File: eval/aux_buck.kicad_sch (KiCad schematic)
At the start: 14 parts, among them U1 AP63205WU-7, U10 TPS7A2033PDBVR, U12 TPS7A2033PDBVR

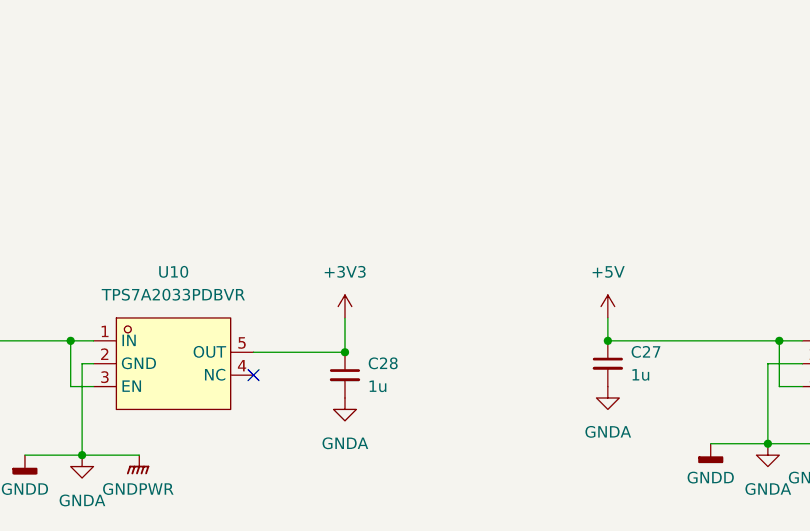
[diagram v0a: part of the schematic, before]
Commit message: [layout] 50*100mm, without trace
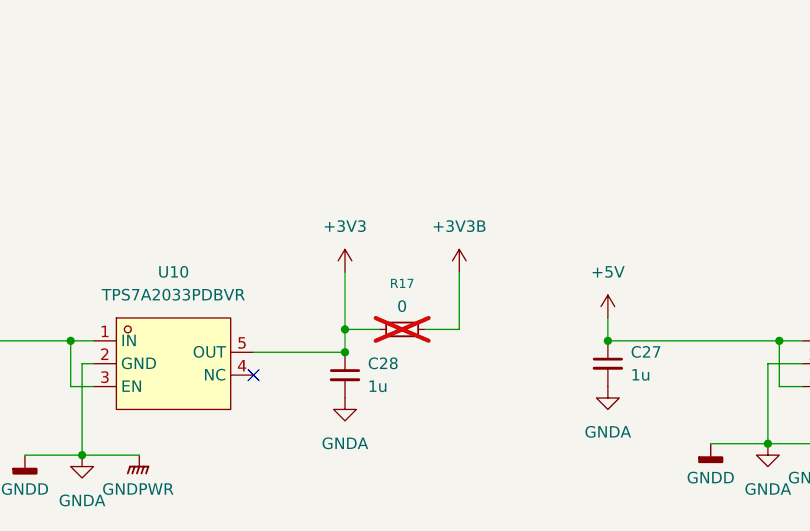
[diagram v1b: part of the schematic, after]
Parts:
- added R17: 0, symbol Device:R_Small
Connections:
- net +3V3: now also R17.1
- net +3V3B: now also R17.2
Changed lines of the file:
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@@
 	)
 	(junction
+		(at 91.44 118.11)
+		(diameter 0)
+		(color 0 0 0 0)
+	)
+	(junction
 		(at 139.7 119.38)
 		(diameter 0)
@@
 	(wire
 		(pts
-			(xy 91.44 116.84) (xy 91.44 120.65)
+			(xy 91.44 111.76) (xy 91.44 118.11)
 		)
 		(stroke
@@
 	(wire
 		(pts
+			(xy 104.14 118.11) (xy 100.33 118.11)
+		)
+		(stroke
+			(width 0)
+			(type default)
+		)
+	)
+	(wire
+		(pts
 			(xy 97.79 60.96) (xy 102.87 60.96)
 		)
@@
 	(wire
 		(pts
+			(xy 104.14 111.76) (xy 104.14 118.11)
+		)
+		(stroke
+			(width 0)
+			(type default)
+		)
+	)
+	(wire
+		(pts
 			(xy 132.08 67.31) (xy 132.08 66.04)
 		)
@@
 	(wire
 		(pts
+			(xy 91.44 118.11) (xy 91.44 120.65)
+		)
+		(stroke
+			(width 0)
+			(type default)
+		)
+	)
+	(wire
+		(pts
 			(xy 102.87 60.96) (xy 105.41 60.96)
 		)
@@
 	(wire
 		(pts
+			(xy 95.25 118.11) (xy 91.44 118.11)
+		)
+		(stroke
+			(width 0)
+			(type default)
+		)
+	)
+	(wire
+		(pts
 			(xy 171.45 120.65) (xy 160.02 120.65)
 		)
@@
 	)
 	(symbol
+		(lib_id "Device:R_Small")
+		(at 97.79 118.11 90)
+		(unit 1)
+		(body_style 1)
+		(exclude_from_sim no)
+		(in_bom yes)
+		(on_board yes)
+		(in_pos_files yes)
+		(dnp yes)
+		(fields_autoplaced yes)
+		(property "Reference" "R17"
+			(at 97.79 113.03 90)
+			(show_name no)
+			(do_not_autoplace no)
+			(effects
+				(font
+					(size 1.016 1.016)
+				)
+			)
+		)
+		(property "Value" "0"
+			(at 97.79 115.57 90)
+			(show_name no)
+			(do_not_autoplace no)
+			(effects
+				(font
+					(size 1.27 1.27)
+				)
+			)
+		)
+		(property "Footprint" ""
+			(at 97.79 118.11 0)
+			(hide yes)
+			(show_name no)
+			(do_not_autoplace no)
+			(effects
+				(font
+					(size 1.27 1.27)
+				)
+			)
+		)
+		(property "Datasheet" ""
+			(at 97.79 118.11 0)
+			(hide yes)
+			(show_name no)
+			(do_not_autoplace no)
+			(effects
+				(font
+					(size 1.27 1.27)
+				)
+			)
+		)
+		(property "Description" "Resistor, small symbol"
+			(at 97.79 118.11 0)
+			(hide yes)
+			(show_name no)
+			(do_not_autoplace no)
+			(effects
+				(font
+					(size 1.27 1.27)
+				)
+			)
+		)
+		(pin "1"
+		)
+		(pin "2"
+		)
+		(instances
+			(project "eval"
+				(path "/8b023652-20db-48ce-ad53-bc2d9a4e5dd4/e5450d34-e34e-454c-8387-40410830d96b"
+					(reference "R17")
+					(unit 1)
+				)
+			)
+		)
+	)
+	(symbol
 		(lib_id "power:+5V")
 		(at 7.1264 11.1816 0)
@@
 	)
 	(symbol
+		(lib_id "power:+3V3")
+		(at 104.14 111.76 0)
+		(unit 1)
+		(body_style 1)
+		(exclude_from_sim no)
+		(in_bom yes)
+		(on_board yes)
+		(in_pos_files yes)
+		(dnp no)
+		(fields_autoplaced yes)
+		(property "Reference" "#PWR0135"
+			(at 104.14 115.57 0)
+			(hide yes)
+			(show_name no)
+			(do_not_autoplace no)
+			(effects
+				(font
+					(size 1.27 1.27)
+				)
+			)
+		)
+		(property "Value" "+3V3B"
+			(at 104.14 106.68 0)
+			(show_name no)
+			(do_not_autoplace no)
+			(effects
+				(font
+					(size 1.27 1.27)
+				)
+			)
+		)
+		(property "Footprint" ""
+			(at 104.14 111.76 0)
+			(hide yes)
+			(show_name no)
+			(do_not_autoplace no)
+			(effects
+				(font
+					(size 1.27 1.27)
+				)
+			)
+		)
+		(property "Datasheet" ""
+			(at 104.14 111.76 0)
+			(hide yes)
+			(show_name no)
+			(do_not_autoplace no)
+			(effects
+				(font
+					(size 1.27 1.27)
+				)
+			)
+		)
+		(property "Description" "Power symbol creates a global label with name \"+3V3\""
+			(at 104.14 111.76 0)
+			(hide yes)
+			(show_name no)
+			(do_not_autoplace no)
+			(effects
+				(font
+					(size 1.27 1.27)
+				)
+			)
+		)
+		(pin "1"
+		)
+		(instances
+			(project "eval"
+				(path "/8b023652-20db-48ce-ad53-bc2d9a4e5dd4/e5450d34-e34e-454c-8387-40410830d96b"
+					(reference "#PWR0135")
+					(unit 1)
+				)
+			)
+		)
+	)
+	(symbol
 		(lib_id "power:VBUS")
 		(at 52.07 53.34 0)
@@
 	(symbol
 		(lib_id "power:+3V3")
-		(at 91.44 116.84 0)
+		(at 91.44 111.76 0)
 		(unit 1)
 		(body_style 1)
@@
 		(fields_autoplaced yes)
 		(property "Reference" "#PWR038"
-			(at 91.44 120.65 0)
+			(at 91.44 115.57 0)
 			(hide yes)
 			(show_name no)
@@
 		)
 		(property "Value" "+3V3"
-			(at 91.44 111.76 0)
+			(at 91.44 106.68 0)
 			(show_name no)
 			(do_not_autoplace no)
@@
 		)
 		(property "Footprint" ""
-			(at 91.44 116.84 0)
+			(at 91.44 111.76 0)
 			(hide yes)
 			(show_name no)
@@
 		)
 		(property "Datasheet" ""
-			(at 91.44 116.84 0)
+			(at 91.44 111.76 0)
 			(hide yes)
 			(show_name no)
@@
 		)
 		(property "Description" "Power symbol creates a global label with name \"+3V3\""
-			(at 91.44 116.84 0)
+			(at 91.44 111.76 0)
 			(hide yes)
 			(show_name no)
